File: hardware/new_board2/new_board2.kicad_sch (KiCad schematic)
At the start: 49 parts, among them CON1 BARREL_JACK, J1 Conn_01x14_Socket, J7 Conn_01x14_Socket, P10 A2, P11 A3, P12 UART, P13 I2C 1, P14 I2C 2, P15 Conn_01x02, P16 Conn_01x02, P17 Conn_01x02, P18 Conn_01x02, P19 Conn_01x02, P20 Conn_01x02, P21 Conn_01x02, P22 Conn_01x02, P3 Conn_01x02, P4 Conn_01x02, P4 D4, P5 Conn_01x02, P6 D6, P7 D7, P8 D8, P9 A1, P9 Conn_01x02, U1 LM2596T-5, U3 ESP32-DEVKITC-32D

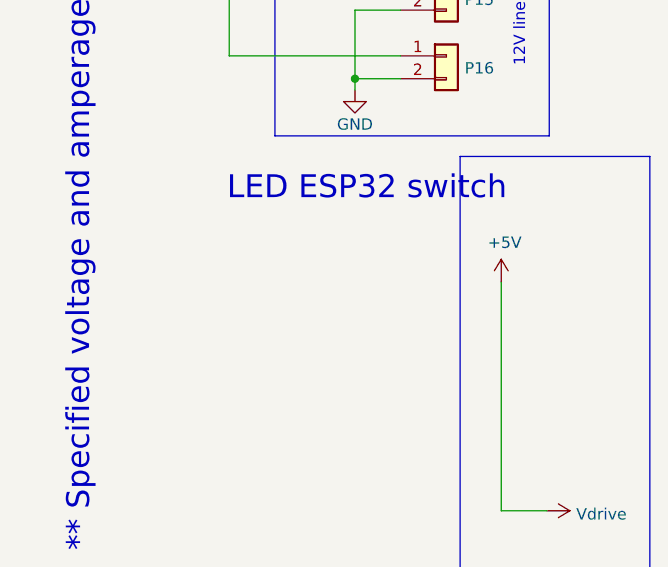
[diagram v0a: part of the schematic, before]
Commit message: pcb version 0.1
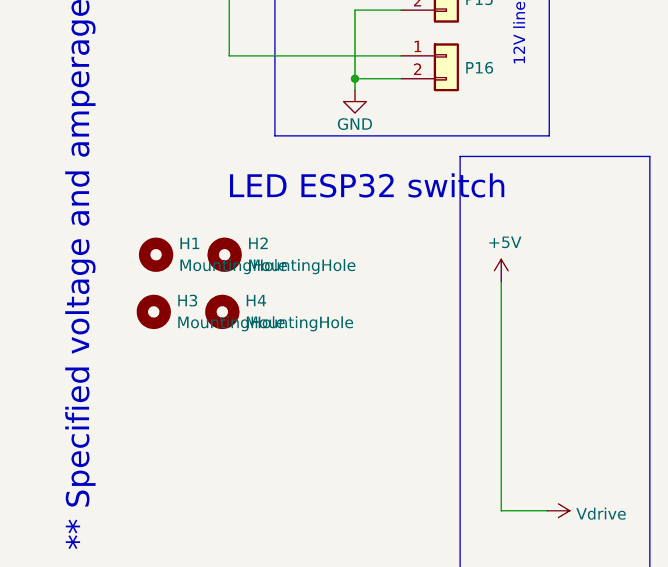
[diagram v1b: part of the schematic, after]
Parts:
- added H1, H2, H3, H4: MountingHole, MountingHole:MountingHole_3.2mm_M3, symbol Mechanical:MountingHole
- P10, P11, P12, P13, P14, P4, P6, P7, P8, P9: footprint Connector_PinSocket_2.54mm:PinSocket_1x02_P2.54mm_Vertical -> Connector_JST:JST_XH_B4B-XH-A_1x04_P2.50mm_Vertical
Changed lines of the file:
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@@
       (effects (font (size 1.27 1.27)))
     )
-    (property "Footprint" "Connector_PinSocket_2.54mm:PinSocket_1x02_P2.54mm_Vertical" (at 235.204 125.476 0)
+    (property "Footprint" "Connector_JST:JST_XH_B4B-XH-A_1x04_P2.50mm_Vertical" (at 235.204 125.476 0)
       (effects (font (size 1.27 1.27)) hide)
     )
@@
   )
   (symbol (lib_id "Connector:Conn_01x14_Socket") (at 539.75 22.606 0) (unit 1)
-    (in_bom yes) (on_board yes) (dnp no) (fields_autoplaced)
+    (in_bom yes) (on_board yes) (dnp no)
     (property "Reference" "J1" (at 540.4612 22.6639 0)
       (effects (font (size 1.27 1.27)) (justify left))
@@
     )
   )
+  (symbol (lib_id "Mechanical:MountingHole") (at 36.576 113.792 0) (unit 1)
+    (in_bom yes) (on_board yes) (dnp no) (fields_autoplaced)
+    (property "Reference" "H2" (at 39.116 112.5799 0)
+      (effects (font (size 1.27 1.27)) (justify left))
+    )
+    (property "Value" "MountingHole" (at 39.116 115.0041 0)
+      (effects (font (size 1.27 1.27)) (justify left))
+    )
+    (property "Footprint" "MountingHole:MountingHole_3.2mm_M3" (at 36.576 113.792 0)
+      (effects (font (size 1.27 1.27)) hide)
+    )
+    (property "Datasheet" "~" (at 36.576 113.792 0)
+      (effects (font (size 1.27 1.27)) hide)
+    )
+    (instances
+      (project "new_board2"
+        (path "/5bd5373d-bd25-4877-850d-beaf1044871d"
+          (reference "H2") (unit 1)
+        )
+      )
+    )
+  )
+  (symbol (lib_id "Mechanical:MountingHole") (at 28.702 120.142 0) (unit 1)
+    (in_bom yes) (on_board yes) (dnp no) (fields_autoplaced)
+    (property "Reference" "H3" (at 31.242 118.9299 0)
+      (effects (font (size 1.27 1.27)) (justify left))
+    )
+    (property "Value" "MountingHole" (at 31.242 121.3541 0)
+      (effects (font (size 1.27 1.27)) (justify left))
+    )
+    (property "Footprint" "MountingHole:MountingHole_3.2mm_M3" (at 28.702 120.142 0)
+      (effects (font (size 1.27 1.27)) hide)
+    )
+    (property "Datasheet" "~" (at 28.702 120.142 0)
+      (effects (font (size 1.27 1.27)) hide)
+    )
+    (instances
+      (project "new_board2"
+        (path "/5bd5373d-bd25-4877-850d-beaf1044871d"
+          (reference "H3") (unit 1)
+        )
+      )
+    )
+  )
   (symbol (lib_id "Device:R") (at 373.634 19.812 90) (unit 1)
     (in_bom yes) (on_board yes) (dnp no)
@@
       (effects (font (size 1.27 1.27)))
     )
-    (property "Footprint" "Connector_PinSocket_2.54mm:PinSocket_1x02_P2.54mm_Vertical" (at 170.434 53.086 0)
+    (property "Footprint" "Connector_JST:JST_XH_B4B-XH-A_1x04_P2.50mm_Vertical" (at 170.434 53.086 0)
       (effects (font (size 1.27 1.27)) hide)
     )
@@
       (effects (font (size 1.27 1.27)))
     )
-    (property "Footprint" "Connector_PinSocket_2.54mm:PinSocket_1x02_P2.54mm_Vertical" (at 146.304 159.766 0)
+    (property "Footprint" "Connector_JST:JST_XH_B4B-XH-A_1x04_P2.50mm_Vertical" (at 146.304 159.766 0)
       (effects (font (size 1.27 1.27)) hide)
     )
@@
     )
   )
+  (symbol (lib_id "Mechanical:MountingHole") (at 36.322 120.142 0) (unit 1)
+    (in_bom yes) (on_board yes) (dnp no) (fields_autoplaced)
+    (property "Reference" "H4" (at 38.862 118.9299 0)
+      (effects (font (size 1.27 1.27)) (justify left))
+    )
+    (property "Value" "MountingHole" (at 38.862 121.3541 0)
+      (effects (font (size 1.27 1.27)) (justify left))
+    )
+    (property "Footprint" "MountingHole:MountingHole_3.2mm_M3" (at 36.322 120.142 0)
+      (effects (font (size 1.27 1.27)) hide)
+    )
+    (property "Datasheet" "~" (at 36.322 120.142 0)
+      (effects (font (size 1.27 1.27)) hide)
+    )
+    (instances
+      (project "new_board2"
+        (path "/5bd5373d-bd25-4877-850d-beaf1044871d"
+          (reference "H4") (unit 1)
+        )
+      )
+    )
+  )
   (symbol (lib_id "Device:R") (at 556.514 102.362 0) (unit 1)
     (in_bom yes) (on_board yes) (dnp no)
@@
       (effects (font (size 1.27 1.27)))
     )
-    (property "Footprint" "Connector_PinSocket_2.54mm:PinSocket_1x02_P2.54mm_Vertical" (at 194.564 125.476 0)
+    (property "Footprint" "Connector_JST:JST_XH_B4B-XH-A_1x04_P2.50mm_Vertical" (at 194.564 125.476 0)
       (effects (font (size 1.27 1.27)) hide)
     )
@@
       (effects (font (size 1.27 1.27)))
     )
-    (property "Footprint" "Connector_PinSocket_2.54mm:PinSocket_1x02_P2.54mm_Vertical" (at 170.434 86.106 0)
+    (property "Footprint" "Connector_JST:JST_XH_B4B-XH-A_1x04_P2.50mm_Vertical" (at 170.434 86.106 0)
       (effects (font (size 1.27 1.27)) hide)
     )
@@
       (effects (font (size 1.27 1.27)))
     )
-    (property "Footprint" "Connector_PinSocket_2.54mm:PinSocket_1x02_P2.54mm_Vertical" (at 170.434 125.476 0)
+    (property "Footprint" "Connector_JST:JST_XH_B4B-XH-A_1x04_P2.50mm_Vertical" (at 170.434 125.476 0)
       (effects (font (size 1.27 1.27)) hide)
     )
@@
     )
   )
+  (symbol (lib_id "Mechanical:MountingHole") (at 28.956 113.792 0) (unit 1)
+    (in_bom yes) (on_board yes) (dnp no) (fields_autoplaced)
+    (property "Reference" "H1" (at 31.496 112.5799 0)
+      (effects (font (size 1.27 1.27)) (justify left))
+    )
+    (property "Value" "MountingHole" (at 31.496 115.0041 0)
+      (effects (font (size 1.27 1.27)) (justify left))
+    )
+    (property "Footprint" "MountingHole:MountingHole_3.2mm_M3" (at 28.956 113.792 0)
+      (effects (font (size 1.27 1.27)) hide)
+    )
+    (property "Datasheet" "~" (at 28.956 113.792 0)
+      (effects (font (size 1.27 1.27)) hide)
+    )
+    (instances
+      (project "new_board2"
+        (path "/5bd5373d-bd25-4877-850d-beaf1044871d"
+          (reference "H1") (unit 1)
+        )
+      )
+    )
+  )
   (symbol (lib_id "power:+12V") (at 39.37 29.718 0) (unit 1)
     (in_bom yes) (on_board yes) (dnp no) (fields_autoplaced)
@@
       (effects (font (size 1.27 1.27)))
     )
-    (property "Footprint" "Connector_PinSocket_2.54mm:PinSocket_1x02_P2.54mm_Vertical" (at 235.204 108.966 0)
+    (property "Footprint" "Connector_JST:JST_XH_B4B-XH-A_1x04_P2.50mm_Vertical" (at 235.204 108.966 0)
       (effects (font (size 1.27 1.27)) hide)
     )
@@
       (effects (font (size 1.27 1.27)))
     )
-    (property "Footprint" "Connector_PinSocket_2.54mm:PinSocket_1x02_P2.54mm_Vertical" (at 146.304 125.476 0)
+    (property "Footprint" "Connector_JST:JST_XH_B4B-XH-A_1x04_P2.50mm_Vertical" (at 146.304 125.476 0)
       (effects (font (size 1.27 1.27)) hide)
     )
@@
       (effects (font (size 1.27 1.27)))
     )
-    (property "Footprint" "Connector_PinSocket_2.54mm:PinSocket_1x02_P2.54mm_Vertical" (at 170.434 69.596 0)
+    (property "Footprint" "Connector_JST:JST_XH_B4B-XH-A_1x04_P2.50mm_Vertical" (at 170.434 69.596 0)
       (effects (font (size 1.27 1.27)) hide)
     )
@@
       (effects (font (size 1.27 1.27)))
     )
-    (property "Footprint" "Connector_PinSocket_2.54mm:PinSocket_1x02_P2.54mm_Vertical" (at 146.304 86.106 0)
-      (effects (font (size 1.27 1.27)) hide)
-    )
+    (property "Footprint" "Connector_JST:JST_XH_B4B-XH-A_1x04_P2.50mm_Vertical" (at 146.304 86.106 0)
+      (effects (font (size 1.27 1.27)) hide)
+    )
